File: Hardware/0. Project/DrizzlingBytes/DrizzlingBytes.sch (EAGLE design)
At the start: 30 parts, among them CN1 USB Type C Receptacle, CN7 JTAG, Q4 NPN-PMMT491, Q5 NPN-PMMT491, U1 MSP430FR4133, U14 CP2102N

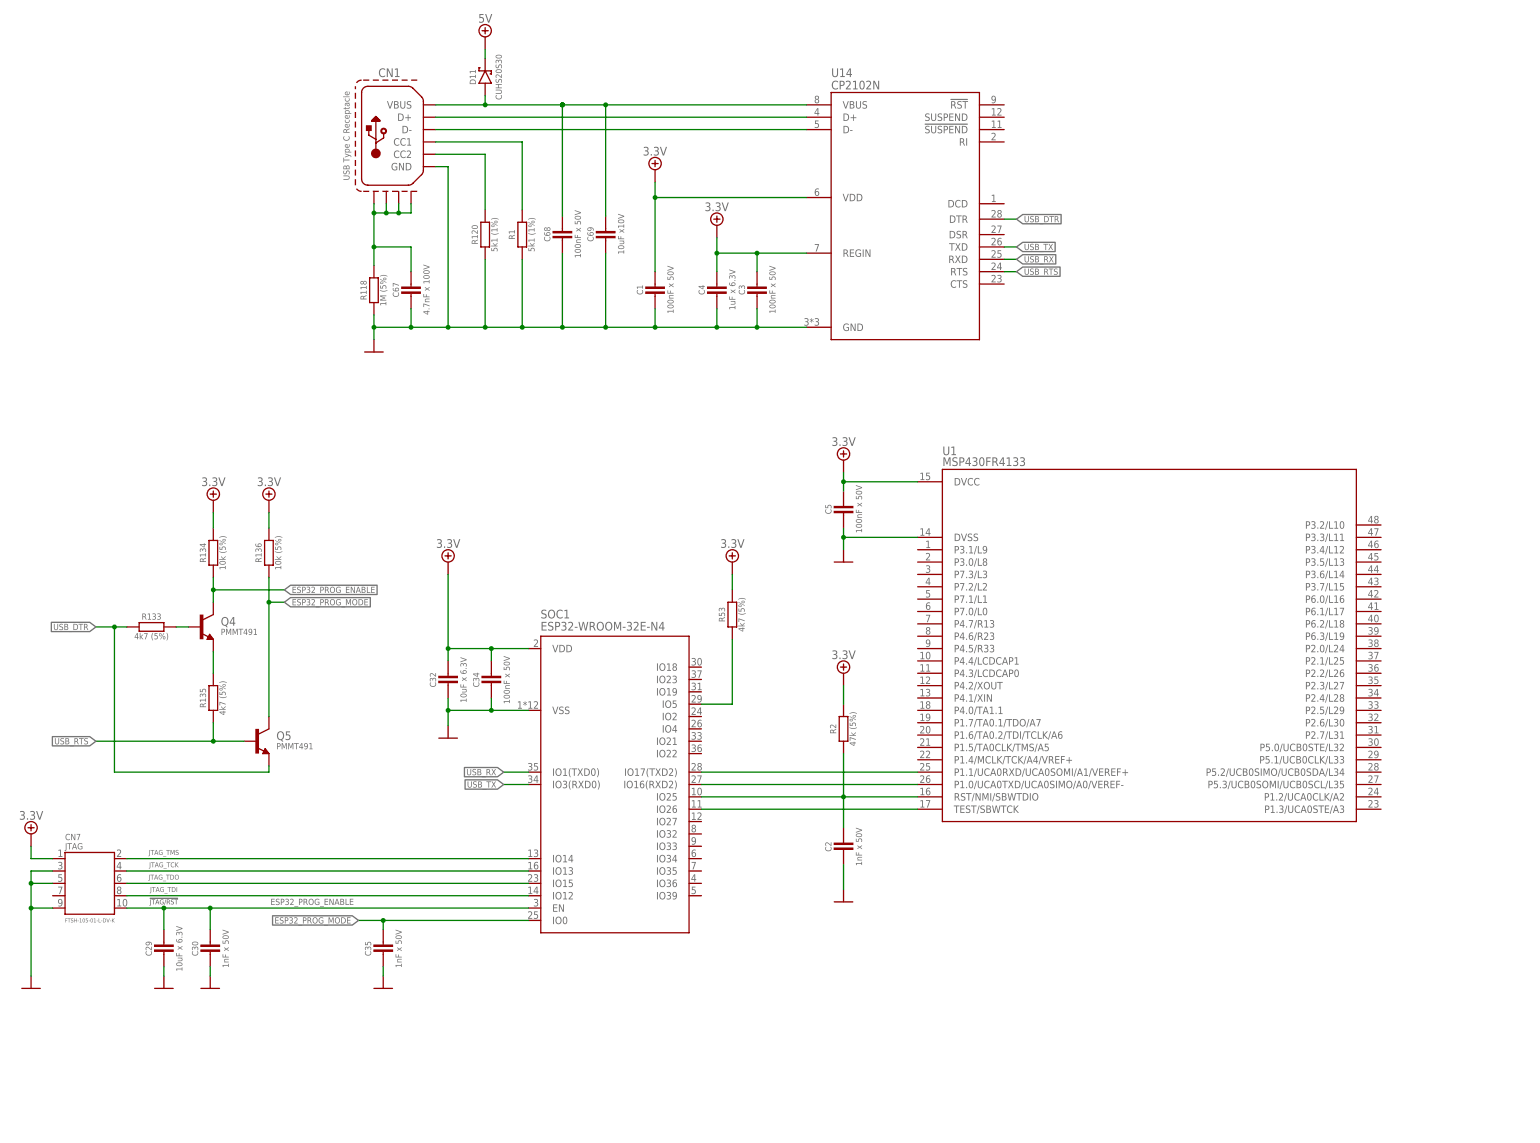
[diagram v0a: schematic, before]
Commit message: WIP
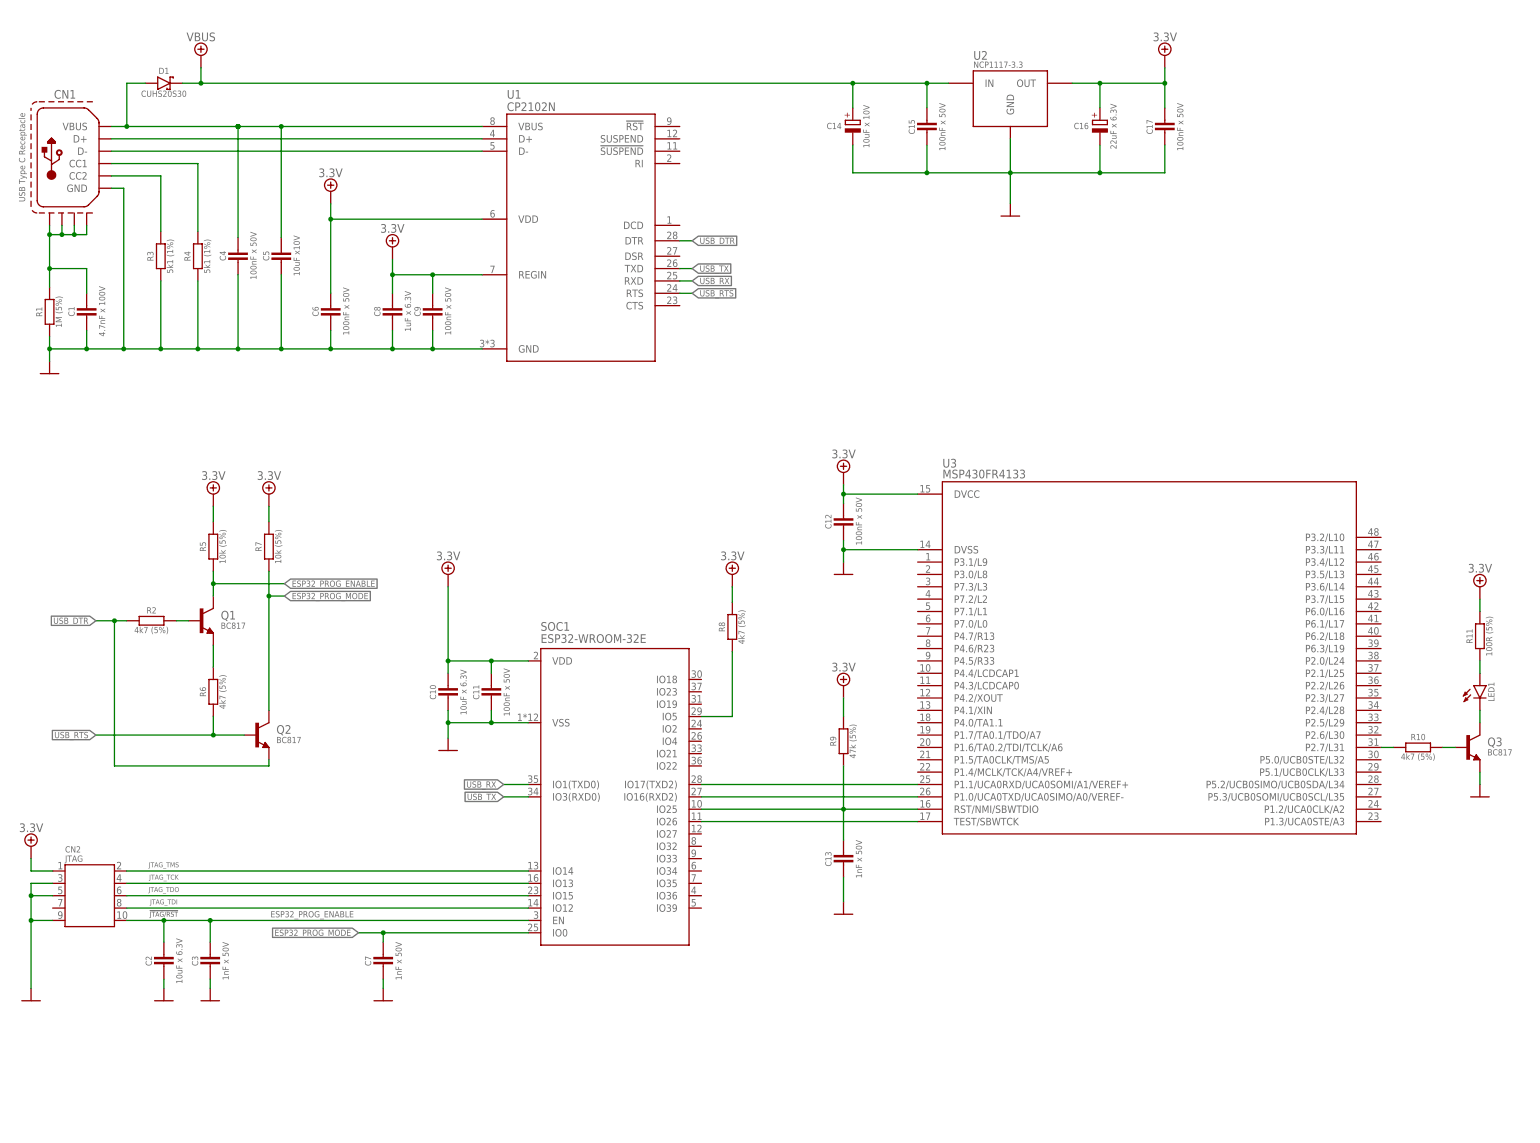
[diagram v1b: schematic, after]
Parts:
- removed C29, C32: 10uF x 6.3V, My-RLC:C_0402
- removed C30, C35: 1nF x 50V, My-RLC:C_0402
- removed C34, C68: 100nF x 50V, My-RLC:C_0402
- removed C67: 4.7nF x 100V, My-RLC:C_0402
- removed C69: 10uF x10V, My-RLC:C_0402
- removed CN7: JTAG, My-Connectors:JTAG
- removed D11: SCHOTTKY-CUHS20S30, My-Diodes:SCHOTTKY-CUHS20S30
- removed Q4, Q5: NPN-PMMT491, My-Transistors:NPN-PMMT491
- removed R118: 1M (5%), My-RLC:R_0402
- removed R120: 5k1 (1%), My-RLC:R_0402
- removed R133, R135, R53: 4k7 (5%), My-RLC:R_0402
- removed R134, R136: 10k (5%), My-RLC:R_0402
- removed U14: CP2102N, My-ICs:CP2102N
- added C10: 10uF x 6.3V, My-RLC:C_0402
- added C11, C12, C15, C17, C6, C9: 100nF x 50V, My-RLC:C_0402
- added C13, C7: 1nF x 50V, My-RLC:C_0402
- added C14: 10uF x 10V, My-RLC:CP_1206_POL
- added C16: 22uF x 6.3V, My-RLC:CP_1206_POL
- added C8: 1uF x 6.3V, My-RLC:C_0402
- added CN2: JTAG, My-Connectors:JTAG
- added D1: SCHOTTKY-CUHS20S30, My-Diodes:SCHOTTKY-CUHS20S30
- added LED1: LED-0402, My-LEDs:LED-0402
- added Q1, Q2, Q3: NPN-BC817, My-Transistors:NPN-BC817
- added R10, R6, R8: 4k7 (5%), My-RLC:R_0402
- added R11: 100R (5%), My-RLC:R_0402
- added R3, R4: 5k1 (1%), My-RLC:R_0402
- added R5, R7: 10k (5%), My-RLC:R_0402
- added R9: 47k (5%), My-RLC:R_0402
- added U2: 1117-3.3V, My-LDOs:1117-3.3V
- added U3: MSP430FR4133, My-Microcontrollers:MSP430FR4133IG48R
- C1: value 100nF x 50V -> 4.7nF x 100V; PN GRM155R61H104KE19D -> (none)
- C2: value 1nF x 50V -> 10uF x 6.3V; PARTNO GRM155R71H104KE14D -> (none); PN GRM155R61H104KE19D -> (none)
- C3: value 100nF x 50V -> 1nF x 50V; PN GRM155R61H104KE19D -> (none)
- C4: value 1uF x 6.3V -> 100nF x 50V; PN GRM155R61H104KE19D -> (none)
- C5: value 100nF x 50V -> 10uF x10V; PARTNO GRM155R71H104KE14D -> (none); PN GRM155R61H104KE19D -> (none)
- R1: value 5k1 (1%) -> 1M (5%); PARTNO AC0402FR-075K1L -> (none); PN ERJ-2RKF5101X -> (none)
- R2: value 47k (5%) -> 4k7 (5%); PARTNO RC0402JR-074K7L -> (none); PN ERJ-2GEJ472X -> (none)
- SOC1: value ESP32-WROOM-32E-N4 -> ESP32-WROOM-32E; PN ESP32-WROOM-32D-N4 -> (none)
- U1: value MSP430FR4133 -> CP2102N; device My-Microcontrollers:MSP430FR4133IG48R -> My-ICs:CP2102N; PN MSP430FR4133 -> (none)
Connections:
- removed net 5.0V: D11.K
- new net N$11: Q3.B, R10.2
- new net N$12: R10.1, U3.P2.7/L31
- new net N$13: LED1.K, Q3.C
- new net N$14: LED1.A, R11.1
- new net VBUS: C14.+, C15.1, D1.K, U2.IN
- net !ESP32_GPIO_ETHERNET_SPI_CS: now also R8.1; no longer R53.1
- net 0V: now also C10.2, C11.2, C12.1, C13.2, C14.-, C15.2, C16.-, C17.2, C3.2, C6.1, C7.2, C8.1, C9.1, CN2.GND, CN2.GND2, CN2.GND3, Q3.E, R3.2, R4.2, U1.GND, U2.GND, U3.DVSS; no longer C29.2, C3.1, C30.2, C32.2, C34.2, C35.2, C67.1, C68.1, C69.1, CN7.GND, CN7.GND2, CN7.GND3, R118.2, R120.2, U1.DVSS, U14.GND
- net 3.3V: now also C10.1, C11.1, C12.2, C16.+, C17.1, C6.2, C8.2, C9.2, CN2.VDD, R11.2, R5.1, R7.1, R8.2, R9.2, U1.REGIN, U1.VDD, U2.OUT, U3.DVCC; no longer C1.2, C3.2, C32.1, C34.1, C4.2, C5.2, CN7.VDD, R134.1, R136.1, R2.2, R53.2, U1.DVCC, U14.REGIN, U14.VDD
- net ESP32_PROG_ENABLE: now also C2.1, C3.1, CN2.!RST, Q1.C, R5.2; no longer C29.1, C30.1, CN7.!RST, Q4.C, R134.2
- net ESP32_PROG_MODE: now also C7.1, Q2.C, R7.2; no longer C35.1, Q5.C, R136.2
- net JTAG_TCK: now also CN2.TCK; no longer CN7.TCK
- net JTAG_TDI: now also CN2.TDI; no longer CN7.TDI
- net JTAG_TDO: now also CN2.TDO; no longer CN7.TDO
- net JTAG_TMS: now also CN2.TMS; no longer CN7.TMS
- net N$1: now also R3.1; no longer R120.1
- net N$10: now also C13.1, R9.1, U3.RST/NMI/SBWTDIO; no longer C2.1, R2.1, U1.RST/NMI/SBWTDIO
- net N$2: now also R4.1; no longer R1.1
- net N$3: now also U3.P1.1/UCA0RXD/UCA0SOMI/A1/VEREF+; no longer U1.P1.1/UCA0RXD/UCA0SOMI/A1/VEREF+
- net N$4: now also C4.2, C5.2, D1.A, U1.VBUS; no longer C68.2, C69.2, D11.A, U14.VBUS
- net N$5: now also U3.P1.0/UCA0TXD/UCA0SIMO/A0/VEREF-; no longer U1.P1.0/UCA0TXD/UCA0SIMO/A0/VEREF-
- net N$6: now also U1.D+; no longer U14.D+
- net N$7: now also Q1.B, R2.1; no longer Q4.B, R133.1
- net N$79: now also C1.2, R1.1; no longer C67.2, R118.1
- net N$8: now also U1.D-; no longer U14.D-
- net N$9: now also U3.TEST/SBWTCK; no longer U1.TEST/SBWTCK
- net USB_DTR: now also Q2.E, R2.2, U1.DTR; no longer Q5.E, R133.2, U14.DTR
- net USB_RTS: now also Q1.E, Q2.B, R6.1, R6.2, U1.RTS; no longer Q4.E, Q5.B, R135.1, R135.2, U14.RTS
- net USB_RX: now also U1.RXD; no longer U14.RXD
- net USB_TX: now also U1.TXD; no longer U14.TXD
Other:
- moved on the sheet: C1, C2, C3, C4, C5, CN1, R1, R2, SOC1

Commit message: WIP
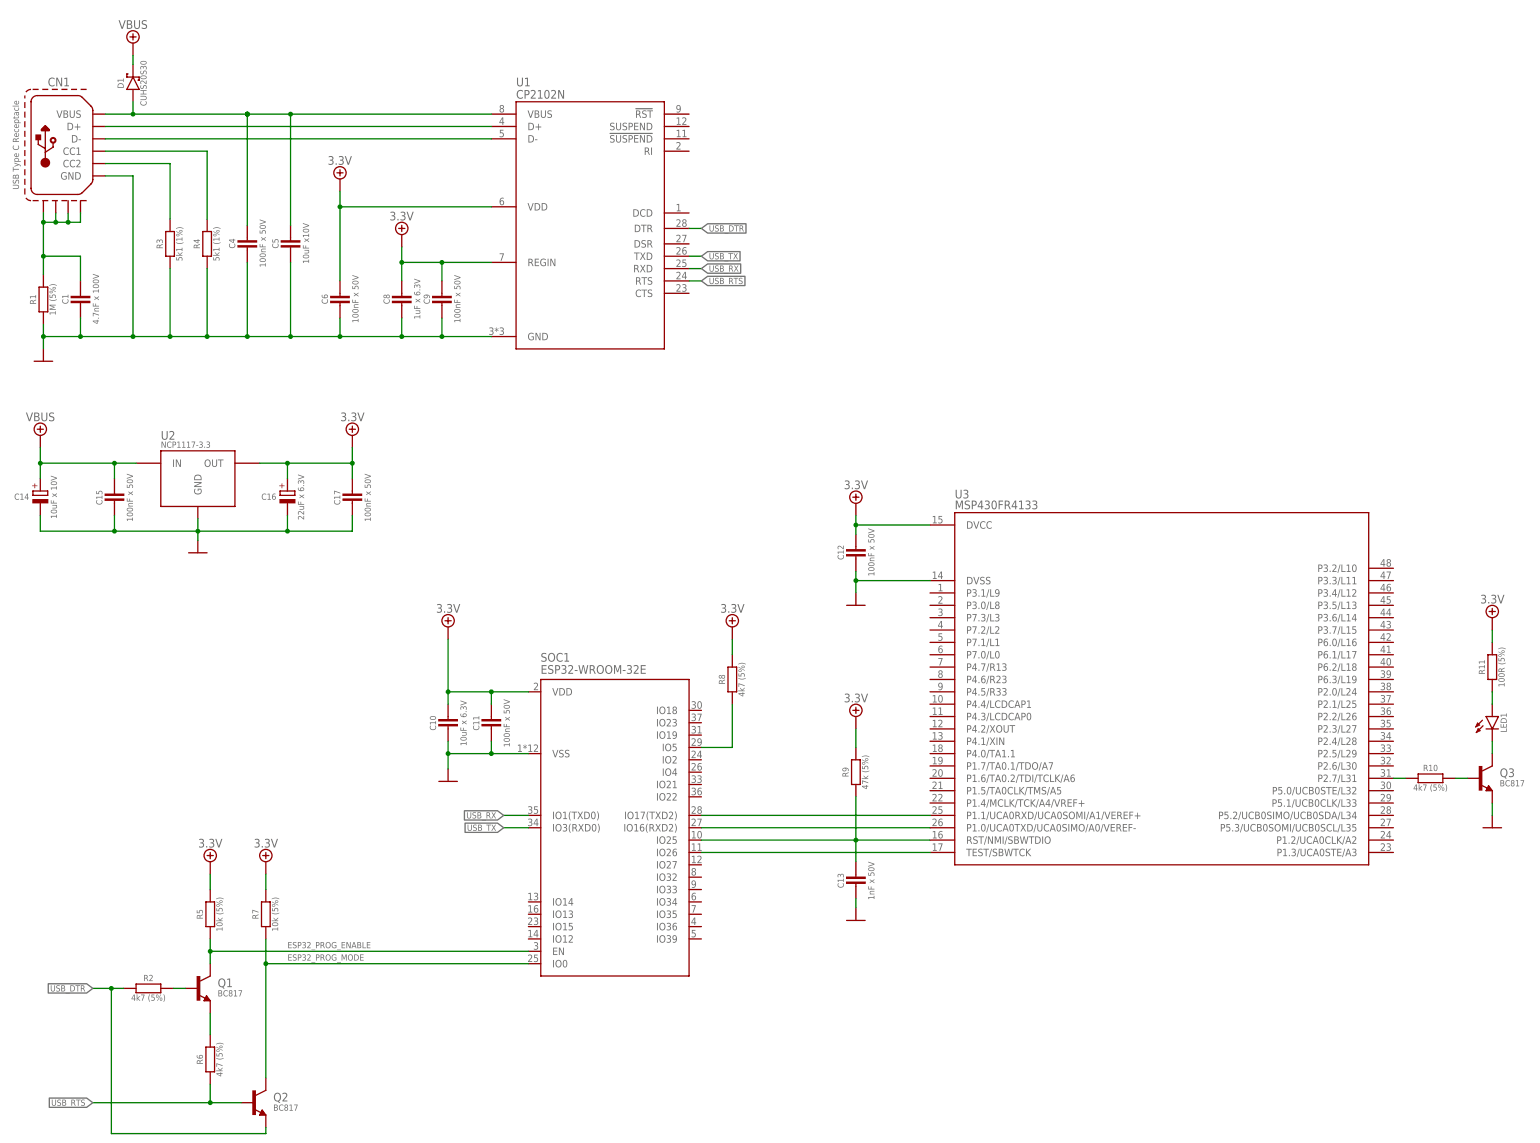
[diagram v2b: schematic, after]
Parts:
- removed C2: 10uF x 6.3V, My-RLC:C_0402
- removed C3, C7: 1nF x 50V, My-RLC:C_0402
- removed CN2: JTAG, My-Connectors:JTAG
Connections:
- removed net JTAG_TCK: CN2.TCK, SOC1.IO13
- removed net JTAG_TDI: CN2.TDI, SOC1.IO12
- removed net JTAG_TDO: CN2.TDO, SOC1.IO15
- removed net JTAG_TMS: CN2.TMS, SOC1.IO14
- net 0V: no longer C2.2, C3.2, C7.2, CN2.GND, CN2.GND2, CN2.GND3
- net 3.3V: no longer CN2.VDD
- net ESP32_PROG_ENABLE: no longer C2.1, C3.1, CN2.!RST
- net ESP32_PROG_MODE: no longer C7.1
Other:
- note added: "ESP32 NodeMCU (Equivalent Circuit)"
- note removed: "!JTAG/RST"
- note removed: "In-Circuit JTAG Programmer and Debugger Interface"
- moved on the sheet: C1, C10, C11, C12, C13, C14, C15, C16, C17, C4, C5, C6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
